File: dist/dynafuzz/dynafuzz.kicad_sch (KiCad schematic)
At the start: 54 parts, among them J1 AudioJack3_Switch, J2 AudioJack3_Switch, J3 Jack-DC, Q1 Q_NPN, Q2 Q_NPN, Q3 Q_NPN, Q4 Q_NPN, SW1 SW_3PDT_x3

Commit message: place fixed elements
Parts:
- D1, D2, D3, D4: footprint Diode_THT:D_A-405_P7.62mm_Horizontal -> Diode_THT:D_A-405_P2.54mm_Vertical_KathodeUp
- R1, R10, R11, R12, R13, R14, R15, R16, R17, R18, R19, R2, R20, R21, R22, R23, R3, R4, R5, R6, R7, R8, R9: footprint Resistor_THT:R_Axial_DIN0207_L6.3mm_D2.5mm_P10.16mm_Horizontal -> Resistor_THT:R_Axial_DIN0207_L6.3mm_D2.5mm_P2.54mm_Vertical
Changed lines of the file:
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@@
 			)
 		)
-		(property "Footprint" "Resistor_THT:R_Axial_DIN0207_L6.3mm_D2.5mm_P10.16mm_Horizontal"
+		(property "Footprint" "Resistor_THT:R_Axial_DIN0207_L6.3mm_D2.5mm_P2.54mm_Vertical"
 			(at 190.5 118.618 90)
 			(effects
@@
 			)
 		)
-		(property "Footprint" "Resistor_THT:R_Axial_DIN0207_L6.3mm_D2.5mm_P10.16mm_Horizontal"
+		(property "Footprint" "Resistor_THT:R_Axial_DIN0207_L6.3mm_D2.5mm_P2.54mm_Vertical"
 			(at 54.102 111.76 90)
 			(effects
@@
 			)
 		)
-		(property "Footprint" "Resistor_THT:R_Axial_DIN0207_L6.3mm_D2.5mm_P10.16mm_Horizontal"
+		(property "Footprint" "Resistor_THT:R_Axial_DIN0207_L6.3mm_D2.5mm_P2.54mm_Vertical"
 			(at 38.1 107.188 90)
 			(effects
@@
 			)
 		)
-		(property "Footprint" "Resistor_THT:R_Axial_DIN0207_L6.3mm_D2.5mm_P10.16mm_Horizontal"
+		(property "Footprint" "Resistor_THT:R_Axial_DIN0207_L6.3mm_D2.5mm_P2.54mm_Vertical"
 			(at 221.742 116.84 90)
 			(effects
@@
 			)
 		)
-		(property "Footprint" "Resistor_THT:R_Axial_DIN0207_L6.3mm_D2.5mm_P10.16mm_Horizontal"
+		(property "Footprint" "Resistor_THT:R_Axial_DIN0207_L6.3mm_D2.5mm_P2.54mm_Vertical"
 			(at 153.67 112.268 90)
 			(effects
@@
 			)
 		)
-		(property "Footprint" "Diode_THT:D_A-405_P7.62mm_Horizontal"
+		(property "Footprint" "Diode_THT:D_A-405_P2.54mm_Vertical_KathodeUp"
 			(at 168.91 91.44 0)
 			(effects
@@
 			)
 		)
-		(property "Footprint" "Resistor_THT:R_Axial_DIN0207_L6.3mm_D2.5mm_P10.16mm_Horizontal"
+		(property "Footprint" "Resistor_THT:R_Axial_DIN0207_L6.3mm_D2.5mm_P2.54mm_Vertical"
 			(at 60.96 100.838 90)
 			(effects
@@
 			)
 		)
-		(property "Footprint" "Resistor_THT:R_Axial_DIN0207_L6.3mm_D2.5mm_P10.16mm_Horizontal"
+		(property "Footprint" "Resistor_THT:R_Axial_DIN0207_L6.3mm_D2.5mm_P2.54mm_Vertical"
 			(at 233.172 93.98 90)
 			(effects
@@
 			)
 		)
-		(property "Footprint" "Diode_THT:D_A-405_P7.62mm_Horizontal"
+		(property "Footprint" "Diode_THT:D_A-405_P2.54mm_Vertical_KathodeUp"
 			(at 125.73 90.17 0)
 			(effects
@@
 			)
 		)
-		(property "Footprint" "Resistor_THT:R_Axial_DIN0207_L6.3mm_D2.5mm_P10.16mm_Horizontal"
+		(property "Footprint" "Resistor_THT:R_Axial_DIN0207_L6.3mm_D2.5mm_P2.54mm_Vertical"
 			(at 116.332 115.57 90)
 			(effects
@@
 			)
 		)
-		(property "Footprint" "Resistor_THT:R_Axial_DIN0207_L6.3mm_D2.5mm_P10.16mm_Horizontal"
+		(property "Footprint" "Resistor_THT:R_Axial_DIN0207_L6.3mm_D2.5mm_P2.54mm_Vertical"
 			(at 65.532 88.9 90)
 			(effects
@@
 			)
 		)
-		(property "Footprint" "Resistor_THT:R_Axial_DIN0207_L6.3mm_D2.5mm_P10.16mm_Horizontal"
+		(property "Footprint" "Resistor_THT:R_Axial_DIN0207_L6.3mm_D2.5mm_P2.54mm_Vertical"
 			(at 208.28 90.678 90)
 			(effects
@@
 			)
 		)
-		(property "Footprint" "Resistor_THT:R_Axial_DIN0207_L6.3mm_D2.5mm_P10.16mm_Horizontal"
+		(property "Footprint" "Resistor_THT:R_Axial_DIN0207_L6.3mm_D2.5mm_P2.54mm_Vertical"
 			(at 127.762 120.65 90)
 			(effects
@@
 			)
 		)
-		(property "Footprint" "Resistor_THT:R_Axial_DIN0207_L6.3mm_D2.5mm_P10.16mm_Horizontal"
+		(property "Footprint" "Resistor_THT:R_Axial_DIN0207_L6.3mm_D2.5mm_P2.54mm_Vertical"
 			(at 233.172 121.92 90)
 			(effects
@@
 			)
 		)
-		(property "Footprint" "Resistor_THT:R_Axial_DIN0207_L6.3mm_D2.5mm_P10.16mm_Horizontal"
+		(property "Footprint" "Resistor_THT:R_Axial_DIN0207_L6.3mm_D2.5mm_P2.54mm_Vertical"
 			(at 110.49 110.998 90)
 			(effects
@@
 			)
 		)
-		(property "Footprint" "Resistor_THT:R_Axial_DIN0207_L6.3mm_D2.5mm_P10.16mm_Horizontal"
+		(property "Footprint" "Resistor_THT:R_Axial_DIN0207_L6.3mm_D2.5mm_P2.54mm_Vertical"
 			(at 170.942 121.92 90)
 			(effects
@@
 			)
 		)
-		(property "Footprint" "Resistor_THT:R_Axial_DIN0207_L6.3mm_D2.5mm_P10.16mm_Horizontal"
+		(property "Footprint" "Resistor_THT:R_Axial_DIN0207_L6.3mm_D2.5mm_P2.54mm_Vertical"
 			(at 87.122 120.65 90)
 			(effects
@@
 			)
 		)
-		(property "Footprint" "Resistor_THT:R_Axial_DIN0207_L6.3mm_D2.5mm_P10.16mm_Horizontal"
+		(property "Footprint" "Resistor_THT:R_Axial_DIN0207_L6.3mm_D2.5mm_P2.54mm_Vertical"
 			(at 65.532 116.84 90)
 			(effects
@@
 			)
 		)
-		(property "Footprint" "Resistor_THT:R_Axial_DIN0207_L6.3mm_D2.5mm_P10.16mm_Horizontal"
+		(property "Footprint" "Resistor_THT:R_Axial_DIN0207_L6.3mm_D2.5mm_P2.54mm_Vertical"
 			(at 123.19 104.648 90)
 			(effects
@@
 			)
 		)
-		(property "Footprint" "Diode_THT:D_A-405_P7.62mm_Horizontal"
+		(property "Footprint" "Diode_THT:D_A-405_P2.54mm_Vertical_KathodeUp"
 			(at 125.73 87.63 0)
 			(effects
@@
 			)
 		)
-		(property "Footprint" "Diode_THT:D_A-405_P7.62mm_Horizontal"
+		(property "Footprint" "Diode_THT:D_A-405_P2.54mm_Vertical_KathodeUp"
 			(at 168.91 88.9 0)
 			(effects
@@
 			)
 		)
-		(property "Footprint" "Resistor_THT:R_Axial_DIN0207_L6.3mm_D2.5mm_P10.16mm_Horizontal"
+		(property "Footprint" "Resistor_THT:R_Axial_DIN0207_L6.3mm_D2.5mm_P2.54mm_Vertical"
 			(at 225.298 97.79 90)
 			(effects
@@
 			)
 		)
-		(property "Footprint" "Resistor_THT:R_Axial_DIN0207_L6.3mm_D2.5mm_P10.16mm_Horizontal"
+		(property "Footprint" "Resistor_THT:R_Axial_DIN0207_L6.3mm_D2.5mm_P2.54mm_Vertical"
 			(at 166.37 105.918 90)
 			(effects
@@
 			)
 		)
-		(property "Footprint" "Resistor_THT:R_Axial_DIN0207_L6.3mm_D2.5mm_P10.16mm_Horizontal"
+		(property "Footprint" "Resistor_THT:R_Axial_DIN0207_L6.3mm_D2.5mm_P2.54mm_Vertical"
 			(at 198.882 44.45 90)
 			(effects
@@
 			)
 		)
-		(property "Footprint" "Resistor_THT:R_Axial_DIN0207_L6.3mm_D2.5mm_P10.16mm_Horizontal"
+		(property "Footprint" "Resistor_THT:R_Axial_DIN0207_L6.3mm_D2.5mm_P2.54mm_Vertical"
 			(at 127.762 78.74 90)
 			(effects
@@
 			)
 		)
-		(property "Footprint" "Resistor_THT:R_Axial_DIN0207_L6.3mm_D2.5mm_P10.16mm_Horizontal"
+		(property "Footprint" "Resistor_THT:R_Axial_DIN0207_L6.3mm_D2.5mm_P2.54mm_Vertical"
 			(at 170.942 80.01 90)
 			(effects
@@
 			)
 		)
-		(property "Footprint" "Resistor_THT:R_Axial_DIN0207_L6.3mm_D2.5mm_P10.16mm_Horizontal"
+		(property "Footprint" "Resistor_THT:R_Axial_DIN0207_L6.3mm_D2.5mm_P2.54mm_Vertical"
 			(at 159.512 116.84 90)
 			(effects

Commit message: update silkscreen
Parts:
- C1, C10, C11, C12, C13, C2, C3, C4, C5, C6, C7, C8, C9: footprint Capacitor_THT:C_Rect_L7.0mm_W2.5mm_P5.00mm -> _project:C
- R1, R10, R11, R12, R13, R14, R15, R16, R17, R18, R19, R2, R20, R21, R22, R23, R3, R4, R5, R6, R7, R8, R9: footprint Resistor_THT:R_Axial_DIN0207_L6.3mm_D2.5mm_P2.54mm_Vertical -> _project:R
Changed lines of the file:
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@@
 			)
 		)
-		(property "Footprint" "Resistor_THT:R_Axial_DIN0207_L6.3mm_D2.5mm_P2.54mm_Vertical"
+		(property "Footprint" "_project:R"
 			(at 190.5 118.618 90)
 			(effects
@@
 			)
 		)
-		(property "Footprint" "Resistor_THT:R_Axial_DIN0207_L6.3mm_D2.5mm_P2.54mm_Vertical"
+		(property "Footprint" "_project:R"
 			(at 54.102 111.76 90)
 			(effects
@@
 			)
 		)
-		(property "Footprint" "Resistor_THT:R_Axial_DIN0207_L6.3mm_D2.5mm_P2.54mm_Vertical"
+		(property "Footprint" "_project:R"
 			(at 38.1 107.188 90)
 			(effects
@@
 			)
 		)
-		(property "Footprint" "Resistor_THT:R_Axial_DIN0207_L6.3mm_D2.5mm_P2.54mm_Vertical"
+		(property "Footprint" "_project:R"
 			(at 221.742 116.84 90)
 			(effects
@@
 			)
 		)
-		(property "Footprint" "Resistor_THT:R_Axial_DIN0207_L6.3mm_D2.5mm_P2.54mm_Vertical"
+		(property "Footprint" "_project:R"
 			(at 153.67 112.268 90)
 			(effects
@@
 			)
 		)
-		(property "Footprint" "Capacitor_THT:C_Rect_L7.0mm_W2.5mm_P5.00mm"
+		(property "Footprint" "_project:C"
 			(at 209.55 111.4552 0)
 			(effects
@@
 			)
 		)
-		(property "Footprint" "Resistor_THT:R_Axial_DIN0207_L6.3mm_D2.5mm_P2.54mm_Vertical"
+		(property "Footprint" "_project:R"
 			(at 60.96 100.838 90)
 			(effects
@@
 			)
 		)
-		(property "Footprint" "Capacitor_THT:C_Rect_L7.0mm_W2.5mm_P5.00mm"
+		(property "Footprint" "_project:C"
 			(at 121.92 87.9348 0)
 			(effects
@@
 			)
 		)
-		(property "Footprint" "Resistor_THT:R_Axial_DIN0207_L6.3mm_D2.5mm_P2.54mm_Vertical"
+		(property "Footprint" "_project:R"
 			(at 233.172 93.98 90)
 			(effects
@@
 			)
 		)
-		(property "Footprint" "Capacitor_THT:C_Rect_L7.0mm_W2.5mm_P5.00mm"
+		(property "Footprint" "_project:C"
 			(at 64.77 94.2848 0)
 			(effects
@@
 			)
 		)
-		(property "Footprint" "Resistor_THT:R_Axial_DIN0207_L6.3mm_D2.5mm_P2.54mm_Vertical"
+		(property "Footprint" "_project:R"
 			(at 116.332 115.57 90)
 			(effects
@@
 			)
 		)
-		(property "Footprint" "Resistor_THT:R_Axial_DIN0207_L6.3mm_D2.5mm_P2.54mm_Vertical"
+		(property "Footprint" "_project:R"
 			(at 65.532 88.9 90)
 			(effects
@@
 			)
 		)
-		(property "Footprint" "Resistor_THT:R_Axial_DIN0207_L6.3mm_D2.5mm_P2.54mm_Vertical"
+		(property "Footprint" "_project:R"
 			(at 208.28 90.678 90)
 			(effects
@@
 			)
 		)
-		(property "Footprint" "Resistor_THT:R_Axial_DIN0207_L6.3mm_D2.5mm_P2.54mm_Vertical"
+		(property "Footprint" "_project:R"
 			(at 127.762 120.65 90)
 			(effects
@@
 			)
 		)
-		(property "Footprint" "Resistor_THT:R_Axial_DIN0207_L6.3mm_D2.5mm_P2.54mm_Vertical"
+		(property "Footprint" "_project:R"
 			(at 233.172 121.92 90)
 			(effects
@@
 			)
 		)
-		(property "Footprint" "Resistor_THT:R_Axial_DIN0207_L6.3mm_D2.5mm_P2.54mm_Vertical"
+		(property "Footprint" "_project:R"
 			(at 110.49 110.998 90)
 			(effects
@@
 			)
 		)
-		(property "Footprint" "Capacitor_THT:C_Rect_L7.0mm_W2.5mm_P5.00mm"
+		(property "Footprint" "_project:C"
 			(at 127 98.0948 0)
 			(effects
@@
 			)
 		)
-		(property "Footprint" "Capacitor_THT:C_Rect_L7.0mm_W2.5mm_P5.00mm"
+		(property "Footprint" "_project:C"
 			(at 81.28 98.0948 0)
 			(effects
@@
 			)
 		)
-		(property "Footprint" "Capacitor_THT:C_Rect_L7.0mm_W2.5mm_P5.00mm"
+		(property "Footprint" "_project:C"
 			(at 201.6252 128.27 0)
 			(effects
@@
 			)
 		)
-		(property "Footprint" "Resistor_THT:R_Axial_DIN0207_L6.3mm_D2.5mm_P2.54mm_Vertical"
+		(property "Footprint" "_project:R"
 			(at 170.942 121.92 90)
 			(effects
@@
 			)
 		)
-		(property "Footprint" "Capacitor_THT:C_Rect_L7.0mm_W2.5mm_P5.00mm"
+		(property "Footprint" "_project:C"
 			(at 104.14 108.2548 0)
 			(effects
@@
 			)
 		)
-		(property "Footprint" "Resistor_THT:R_Axial_DIN0207_L6.3mm_D2.5mm_P2.54mm_Vertical"
+		(property "Footprint" "_project:R"
 			(at 87.122 120.65 90)
 			(effects
@@
 			)
 		)
-		(property "Footprint" "Resistor_THT:R_Axial_DIN0207_L6.3mm_D2.5mm_P2.54mm_Vertical"
+		(property "Footprint" "_project:R"
 			(at 65.532 116.84 90)
 			(effects
@@
 			)
 		)
-		(property "Footprint" "Resistor_THT:R_Axial_DIN0207_L6.3mm_D2.5mm_P2.54mm_Vertical"
+		(property "Footprint" "_project:R"
 			(at 123.19 104.648 90)
 			(effects
@@
 			)
 		)
-		(property "Footprint" "Resistor_THT:R_Axial_DIN0207_L6.3mm_D2.5mm_P2.54mm_Vertical"
+		(property "Footprint" "_project:R"
 			(at 225.298 97.79 90)
 			(effects
@@
 			)
 		)
-		(property "Footprint" "Capacitor_THT:C_Rect_L7.0mm_W2.5mm_P5.00mm"
+		(property "Footprint" "_project:C"
 			(at 165.1 89.2048 0)
 			(effects
@@
 			)
 		)
-		(property "Footprint" "Resistor_THT:R_Axial_DIN0207_L6.3mm_D2.5mm_P2.54mm_Vertical"
+		(property "Footprint" "_project:R"
 			(at 166.37 105.918 90)
 			(effects
@@
 			)
 		)
-		(property "Footprint" "Resistor_THT:R_Axial_DIN0207_L6.3mm_D2.5mm_P2.54mm_Vertical"
+		(property "Footprint" "_project:R"
 			(at 198.882 44.45 90)
 			(effects
@@
 			)
 		)
-		(property "Footprint" "Capacitor_THT:C_Rect_L7.0mm_W2.5mm_P5.00mm"
+		(property "Footprint" "_project:C"
 			(at 147.32 109.5248 0)
 			(effects
@@
 			)
 		)
-		(property "Footprint" "Resistor_THT:R_Axial_DIN0207_L6.3mm_D2.5mm_P2.54mm_Vertical"
+		(property "Footprint" "_project:R"
 			(at 127.762 78.74 90)
 			(effects
@@
 			)
 		)
-		(property "Footprint" "Capacitor_THT:C_Rect_L7.0mm_W2.5mm_P5.00mm"
+		(property "Footprint" "_project:C"
 			(at 52.07 104.4448 0)
 			(effects
@@
 			)
 		)
-		(property "Footprint" "Capacitor_THT:C_Rect_L7.0mm_W2.5mm_P5.00mm"
+		(property "Footprint" "_project:C"
 			(at 248.92 103.1748 0)
 			(effects
@@
 			)
 		)
-		(property "Footprint" "Resistor_THT:R_Axial_DIN0207_L6.3mm_D2.5mm_P2.54mm_Vertical"
+		(property "Footprint" "_project:R"
 			(at 170.942 80.01 90)
 			(effects
@@
 			)
 		)
-		(property "Footprint" "Capacitor_THT:C_Rect_L7.0mm_W2.5mm_P5.00mm"
+		(property "Footprint" "_project:C"
 			(at 186.69 105.1052 0)
 			(effects
@@
 			)
 		)
-		(property "Footprint" "Capacitor_THT:C_Rect_L7.0mm_W2.5mm_P5.00mm"
+		(property "Footprint" "_project:C"
 			(at 170.18 99.3648 0)
 			(effects
@@
 			)
 		)
-		(property "Footprint" "Resistor_THT:R_Axial_DIN0207_L6.3mm_D2.5mm_P2.54mm_Vertical"
+		(property "Footprint" "_project:R"
 			(at 159.512 116.84 90)
 			(effects

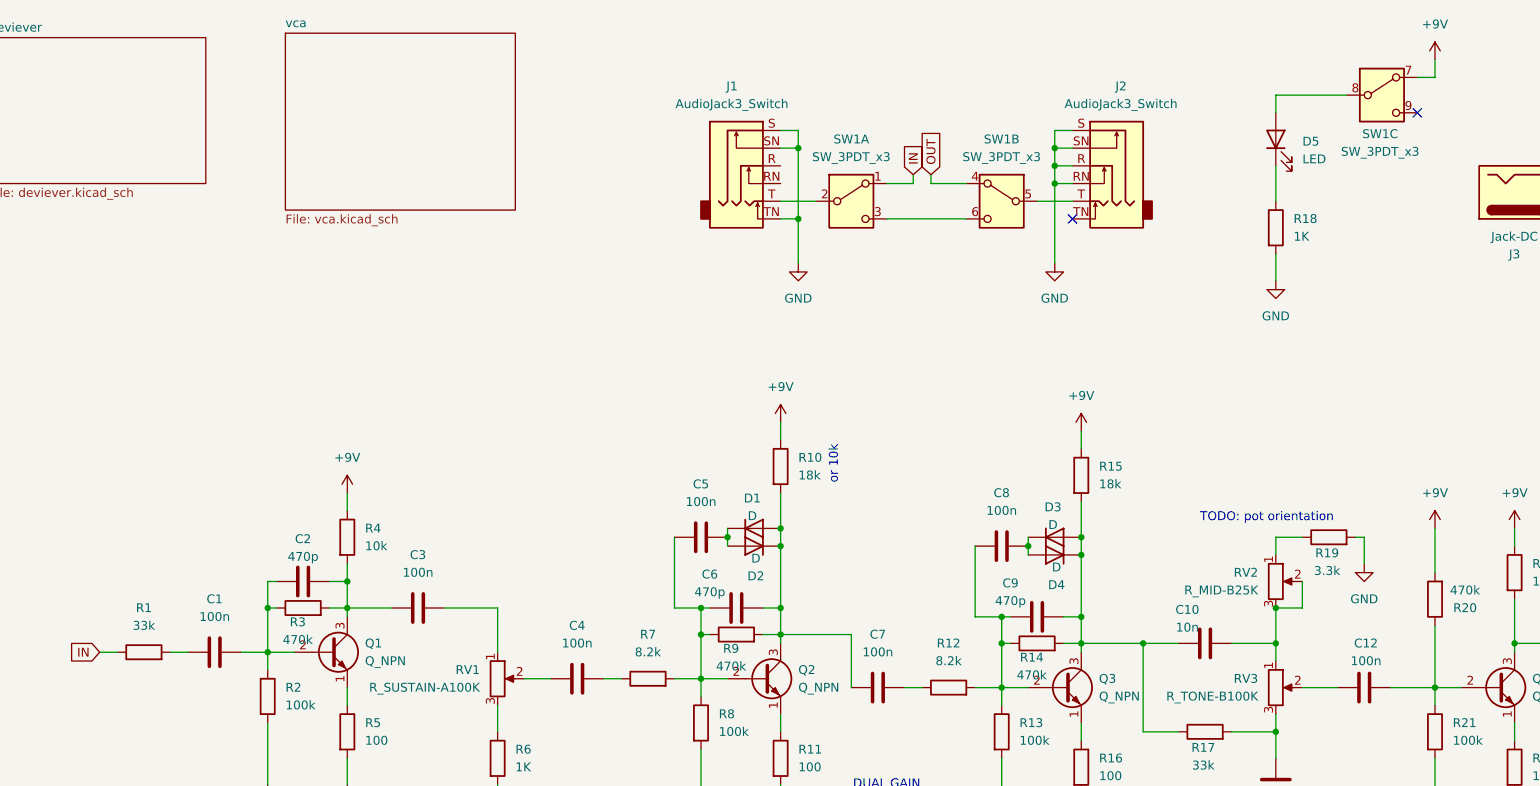
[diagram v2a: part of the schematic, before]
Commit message: layout stage 2 and 3
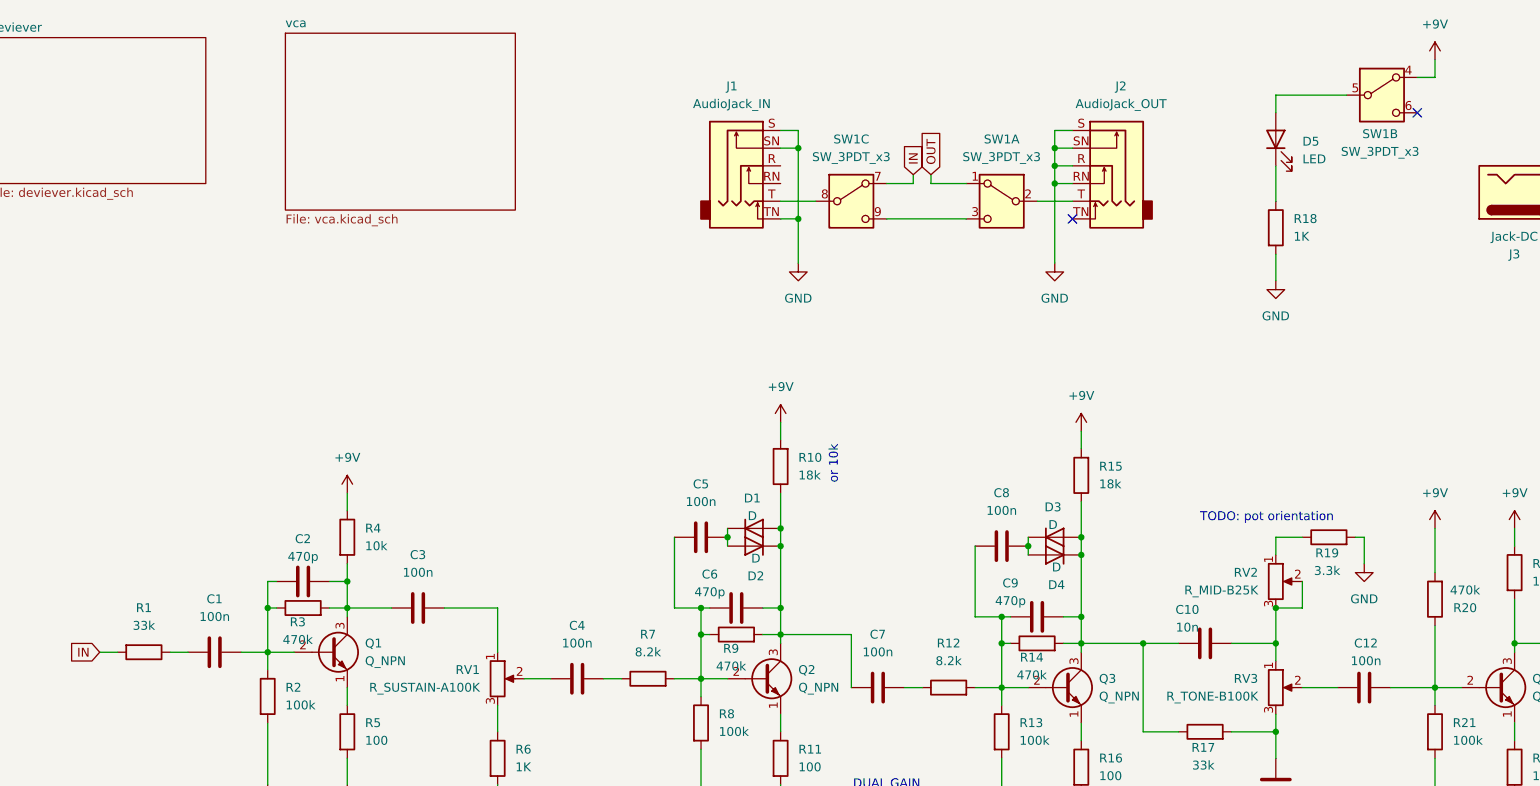
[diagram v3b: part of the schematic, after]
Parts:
- J1: value AudioJack3_Switch -> AudioJack_IN
- J2: value AudioJack3_Switch -> AudioJack_OUT
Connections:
- net +9V: now also R10.2, R15.2, SW1.4 (A); no longer R10.1, R15.1, SW1.7 (A)
- net IN: now also R1.2, SW1.7 (A); no longer R1.1, SW1.1 (A)
- net OUT: now also SW1.1 (A); no longer SW1.4 (A)
- net at C10.2, C9.2, D3.2 (A)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: now also R15.1; no longer R15.2
- net at C1.1: now also R1.1; no longer R1.2
- net at D5.2 (A): now also SW1.5 (B); no longer SW1.8 (B)
- net at J1.T: now also SW1.8 (B); no longer SW1.2 (B)
- net at C6.2, C7.1, D1.2 (A)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: now also R10.1; no longer R10.2
- net at J2.T: now also SW1.2 (B); no longer SW1.5 (B)
- new net: SW1.3 (C), SW1.9 (C)
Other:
- moved on the sheet: R1, R10, R15
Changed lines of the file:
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@@
 	(symbol
 		(lib_id "Device:R")
-		(at 38.1 105.41 90)
+		(at 38.1 105.41 270)
 		(unit 1)
 		(exclude_from_sim no)
@@
 		)
 		(property "Footprint" "_project:R"
-			(at 38.1 107.188 90)
+			(at 38.1 103.632 90)
 			(effects
 				(font
@@
 		(lib_id "_project:SW_3PDT_x3")
 		(at 139.7 40.64 0)
-		(unit 1)
+		(unit 3)
 		(exclude_from_sim no)
 		(in_bom yes)
@@
 				(path "/b401260a-0de9-4b23-a692-63e5f9163375"
 					(reference "SW1")
-					(unit 1)
+					(unit 3)
 				)
 			)
@@
 		(at 161.29 40.64 0)
 		(mirror y)
-		(unit 2)
+		(unit 1)
 		(exclude_from_sim no)
 		(in_bom yes)
@@
 				(path "/b401260a-0de9-4b23-a692-63e5f9163375"
 					(reference "SW1")
-					(unit 2)
+					(unit 1)
 				)
 			)
@@
 			)
 		)
-		(property "Value" "AudioJack3_Switch"
+		(property "Value" "AudioJack_OUT"
 			(at 178.435 26.67 0)
 			(effects
@@
 	(symbol
 		(lib_id "Device:R")
-		(at 129.54 78.74 0)
+		(at 129.54 78.74 180)
 		(unit 1)
 		(exclude_from_sim no)
@@
 					(size 1.27 1.27)
 				)
-				(justify left)
+				(justify right)
 			)
 		)
@@
 					(size 1.27 1.27)
 				)
-				(justify left)
+				(justify right)
 			)
 		)
 		(property "Footprint" "_project:R"
-			(at 127.762 78.74 90)
+			(at 131.318 78.74 90)
 			(effects
 				(font
@@
 	(symbol
 		(lib_id "Device:R")
-		(at 172.72 80.01 0)
+		(at 172.72 80.01 180)
 		(unit 1)
 		(exclude_from_sim no)
@@
 					(size 1.27 1.27)
 				)
-				(justify left)
+				(justify right)
 			)
 		)
@@
 					(size 1.27 1.27)
 				)
-				(justify left)
+				(justify right)
 			)
 		)
 		(property "Footprint" "_project:R"
-			(at 170.942 80.01 90)
+			(at 174.498 80.01 90)
 			(effects
 				(font
@@
 			)
 		)
-		(property "Value" "AudioJack3_Switch"
+		(property "Value" "AudioJack_IN"
 			(at 122.555 26.67 0)
 			(effects
@@
 		(lib_id "_project:SW_3PDT_x3")
 		(at 215.9 25.4 0)
-		(unit 3)
+		(unit 2)
 		(exclude_from_sim no)
 		(in_bom yes)
@@
 				(path "/b401260a-0de9-4b23-a692-63e5f9163375"
 					(reference "SW1")
-					(unit 3)
+					(unit 2)
 				)
 			)
